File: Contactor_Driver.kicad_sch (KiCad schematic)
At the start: 22 parts, among them J9 Conn_01x04, Q1 NMOS, Q8 BUK9M23-80E, Q9 BUK9M23-80E, U5 SI8261ABC-IS

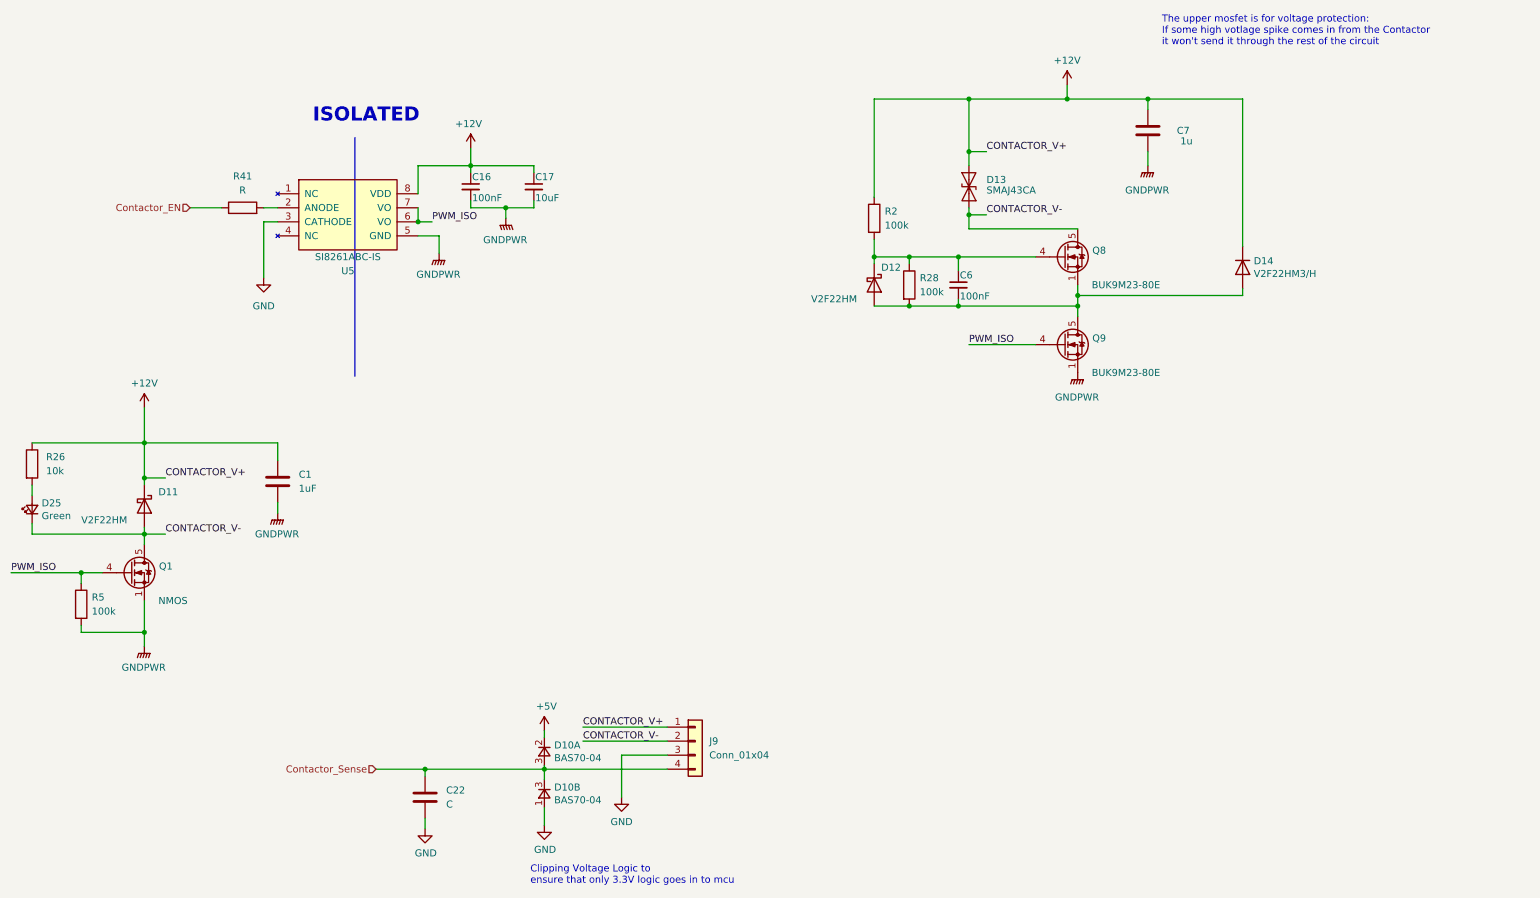
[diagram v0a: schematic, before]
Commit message: New Contactor mosfet
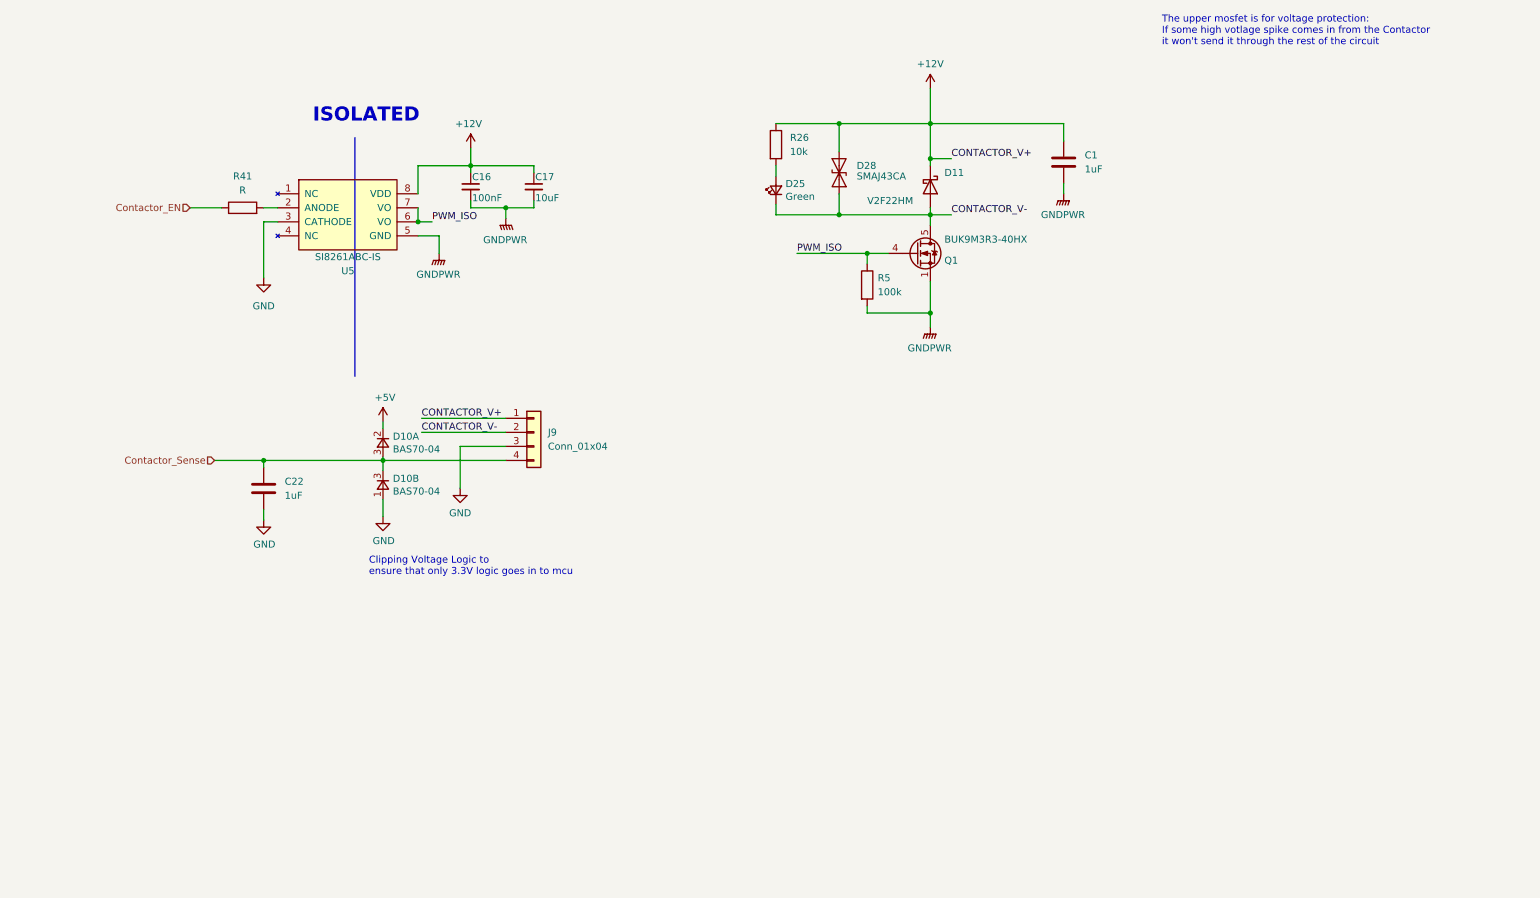
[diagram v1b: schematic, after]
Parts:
- removed C6: 100nF, Capacitor_SMD:C_0805_2012Metric, symbol Device:C_Small
- removed C7: 1u, Capacitor_SMD:C_0805_2012Metric, symbol Device:C
- removed D12: V2F22HM, UTSVT_Passive:V2F22HM, symbol Diode:C3D25170H
- removed D13: SMAJ43CA, Diode_SMD:D_SOD-923, symbol Diode:SZESD9B5.0ST5G
- removed D14: V2F22HM3/H, UTSVT_Passive:V2F22HM, symbol Device:D
- removed Q8, Q9: BUK9M23-80E, Package_TO_SOT_SMD:LFPAK33, symbol Transistor_FET:BUK9M23-80EX
- removed R2, R28: 100k, Resistor_SMD:R_0805_2012Metric, symbol Device:R
- added D28: SMAJ43CA, Diode_SMD:D_SOD-923, symbol Diode:SZESD9B5.0ST5G
- C1: footprint (none) -> Capacitor_SMD:C_0805_2012Metric
- C22: value C -> 1uF; footprint (none) -> Capacitor_SMD:C_0805_2012Metric
- D25: P/N APTD2012LCGCK -> LHR971-KN1
- Q1: value NMOS -> BUK9M3R3-40HX; P/n (none) -> BUK9M3R3-40HX
- R26: footprint (none) -> Resistor_SMD:R_0805_2012Metric
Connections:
- net +12V: now also D28.2 (A2)
- net CONTACTOR_V-: now also D28.1 (A1)
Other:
- moved on the sheet: C1, C22, D10A, D10B, D11, D25, J9, R26, R5
